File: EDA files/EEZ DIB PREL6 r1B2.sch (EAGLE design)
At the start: 65 parts, among them IC1 STM32F030C6T6, IC2 74HC1G126GW,125, IC3 M24C32-WMN6P, IC4 LP2985-33DBVR, K1 RT424005, K2 RT424005, K3 RT424005, K4 RT424005, K5 RT424005, K6 RT424005, Q1 2N7002, Q2 2N7002, Q3 2N7002, Q4 2N7002, Q5 2N7002, Q6 2N7002, X1 SSW-106-02-S-S, X2 77317-104-28LF, X3 691327310016, X4 691327310016

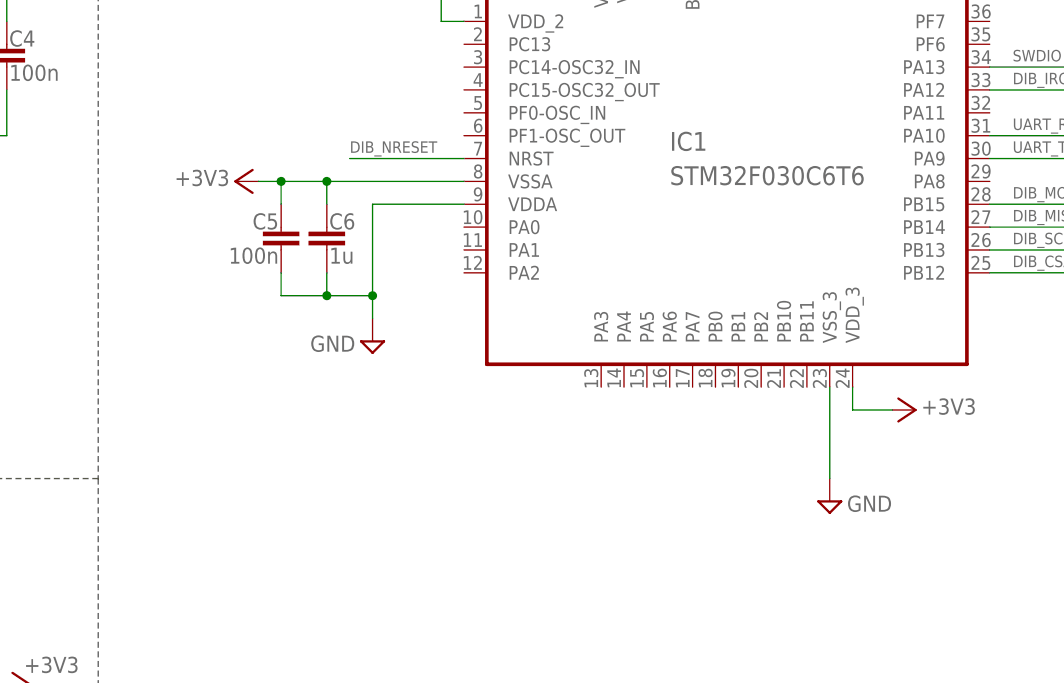
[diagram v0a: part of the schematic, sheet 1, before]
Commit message: #1 fixed
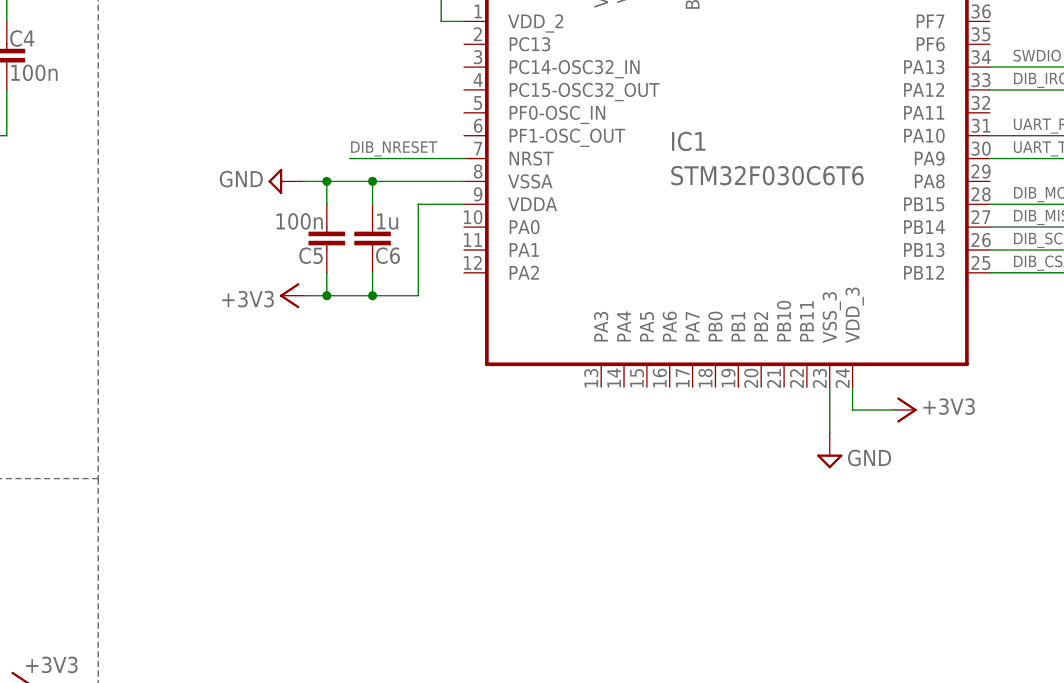
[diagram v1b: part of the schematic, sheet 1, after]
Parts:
- C2, C8, C9: device rcl:C-EUC1206 -> rcl:C-EUC0805
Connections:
- net +3V3: now also IC1.VDDA; no longer IC1.VSSA
- net GND: now also IC1.VSSA; no longer IC1.VDDA
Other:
- moved on the sheet: C5, C6
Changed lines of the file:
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@@
 <part name="SUPPLY66" library="supply2" deviceset="GND" device=""/>
 <part name="SUPPLY67" library="supply2" deviceset="GND" device=""/>
-<part name="C8" library="rcl" deviceset="C-EU" device="C1206" value="2u2"/>
+<part name="C8" library="rcl" deviceset="C-EU" device="C0805" value="2u2"/>
 <part name="P+1" library="supply1" deviceset="+5V" device=""/>
 <part name="P+2" library="supply1" deviceset="+5V" device=""/>
@@
 <part name="P+5" library="supply1" deviceset="+5V" device=""/>
 <part name="IC1" library="EEZ_DIB" deviceset="STM32F030" device="C6T6"/>
-<part name="SUPPLY48" library="supply2" deviceset="GND" device=""/>
 <part name="SUPPLY49" library="supply2" deviceset="GND" device=""/>
 <part name="C1" library="rcl" deviceset="C-EU" device="C0603" value="100n"/>
-<part name="C2" library="rcl" deviceset="C-EU" device="C1206" value="4u7"/>
+<part name="C2" library="rcl" deviceset="C-EU" device="C0805" value="4u7"/>
 <part name="SUPPLY61" library="supply2" deviceset="GND" device=""/>
 <part name="+3V4" library="supply1" deviceset="+3V3" device=""/>
@@
 <part name="C3" library="EEZ_Lib1" deviceset="ECAP" device="PANASONIC_H" value="EEEFK1V470P"/>
 <part name="SUPPLY45" library="supply2" deviceset="GND" device=""/>
-<part name="C9" library="rcl" deviceset="C-EU" device="C1206" value="4u7"/>
+<part name="C9" library="rcl" deviceset="C-EU" device="C0805" value="4u7"/>
 <part name="RN2" library="EEZ_Lib1" deviceset="R_ARRAY4" device="" value="DR1206-10K-4/8"/>
 <part name="+3V5" library="supply1" deviceset="+3V3" device=""/>
@@
 <part name="R7" library="rcl" deviceset="R-EU_" device="R0805" value="100K"/>
 <part name="X1" library="con-samtec" deviceset="SSW-106-02-S-S" device=""/>
+<part name="SUPPLY6" library="supply2" deviceset="GND" device=""/>
 </parts>
 <sheets>
@@
 <attribute name="VALUE" x="205.74" y="98.6536" size="2.0828" layer="96" ratio="6" rot="SR0"/>
 </instance>
-<instance part="SUPPLY48" gate="GND" x="172.72" y="81.28" smashed="yes">
-<attribute name="VALUE" x="170.815" y="81.915" size="1.778" layer="96" rot="R180"/>
-</instance>
-<instance part="SUPPLY49" gate="GND" x="223.52" y="63.5" smashed="yes">
-<attribute name="VALUE" x="225.425" y="64.135" size="1.778" layer="96" rot="MR180"/>
+<instance part="SUPPLY49" gate="GND" x="223.52" y="68.58" smashed="yes">
+<attribute name="VALUE" x="225.425" y="69.215" size="1.778" layer="96" rot="MR180"/>
 </instance>
 <instance part="C1" gate="G$1" x="195.58" y="144.78" smashed="yes" rot="MR90">
@@
 <attribute name="VALUE" x="248.285" y="140.335" size="1.778" layer="96" rot="MR180"/>
 </instance>
-<instance part="C6" gate="G$1" x="167.64" y="91.44" smashed="yes" rot="MR180">
-<attribute name="NAME" x="167.894" y="93.726" size="1.778" layer="95"/>
-<attribute name="VALUE" x="167.894" y="89.916" size="1.778" layer="96"/>
-</instance>
-<instance part="C5" gate="G$1" x="162.56" y="93.98" smashed="yes" rot="MR0">
-<attribute name="NAME" x="162.306" y="93.726" size="1.778" layer="95" rot="MR0"/>
-<attribute name="VALUE" x="162.306" y="89.916" size="1.778" layer="96" rot="MR0"/>
-</instance>
-<instance part="+3V2" gate="G$1" x="157.48" y="99.06" smashed="yes" rot="MR270">
-<attribute name="VALUE" x="156.845" y="100.33" size="1.778" layer="96" rot="R180"/>
+<instance part="C6" gate="G$1" x="172.72" y="93.98" smashed="yes">
+<attribute name="NAME" x="172.974" y="91.694" size="1.778" layer="95" rot="MR180"/>
+<attribute name="VALUE" x="172.974" y="95.504" size="1.778" layer="96" rot="MR180"/>
+</instance>
+<instance part="C5" gate="G$1" x="167.64" y="91.44" smashed="yes" rot="R180">
+<attribute name="NAME" x="167.386" y="91.694" size="1.778" layer="95" rot="R180"/>
+<attribute name="VALUE" x="167.386" y="95.504" size="1.778" layer="96" rot="R180"/>
+</instance>
+<instance part="+3V2" gate="G$1" x="162.56" y="86.36" smashed="yes" rot="R90">
+<attribute name="VALUE" x="161.925" y="85.09" size="1.778" layer="96" rot="MR0"/>
 </instance>
 <instance part="+3V3" gate="G$1" x="233.045" y="73.66" smashed="yes" rot="MR90">
@@
 <instance part="X1" gate="-4" x="177.8" y="165.1" smashed="yes" rot="MR0">
 <attribute name="NAME" x="180.848" y="165.862" size="1.524" layer="95" rot="MR180"/>
+</instance>
+<instance part="SUPPLY6" gate="GND" x="162.56" y="99.06" smashed="yes" rot="MR90">
+<attribute name="VALUE" x="160.655" y="98.425" size="1.778" layer="96" rot="MR0"/>
 </instance>
 </instances>
@@
 </segment>
 <segment>
-<pinref part="IC1" gate="G$1" pin="VDDA"/>
-<wire x1="182.88" y1="96.52" x2="172.72" y2="96.52" width="0.1524" layer="91"/>
-<wire x1="172.72" y1="96.52" x2="172.72" y2="86.36" width="0.1524" layer="91"/>
-<pinref part="SUPPLY48" gate="GND" pin="GND"/>
 <pinref part="C6" gate="G$1" pin="1"/>
-<wire x1="172.72" y1="86.36" x2="172.72" y2="83.82" width="0.1524" layer="91"/>
-<wire x1="172.72" y1="86.36" x2="167.64" y2="86.36" width="0.1524" layer="91"/>
-<wire x1="167.64" y1="86.36" x2="167.64" y2="88.9" width="0.1524" layer="91"/>
-<junction x="172.72" y="86.36"/>
+<wire x1="172.72" y1="99.06" x2="172.72" y2="96.52" width="0.1524" layer="91"/>
 <pinref part="C5" gate="G$1" pin="2"/>
-<wire x1="167.64" y1="86.36" x2="162.56" y2="86.36" width="0.1524" layer="91"/>
-<wire x1="162.56" y1="86.36" x2="162.56" y2="88.9" width="0.1524" layer="91"/>
-<junction x="167.64" y="86.36"/>
+<wire x1="172.72" y1="99.06" x2="167.64" y2="99.06" width="0.1524" layer="91"/>
+<wire x1="167.64" y1="99.06" x2="167.64" y2="96.52" width="0.1524" layer="91"/>
+<junction x="172.72" y="99.06"/>
+<pinref part="IC1" gate="G$1" pin="VSSA"/>
+<wire x1="172.72" y1="99.06" x2="182.88" y2="99.06" width="0.1524" layer="91"/>
+<pinref part="SUPPLY6" gate="GND" pin="GND"/>
+<wire x1="167.64" y1="99.06" x2="165.1" y2="99.06" width="0.1524" layer="91"/>
+<junction x="167.64" y="99.06"/>
 </segment>
 <segment>
 <pinref part="IC1" gate="G$1" pin="VSS_3"/>
-<wire x1="223.52" y1="76.2" x2="223.52" y2="66.04" width="0.1524" layer="91"/>
+<wire x1="223.52" y1="76.2" x2="223.52" y2="71.12" width="0.1524" layer="91"/>
 <pinref part="SUPPLY49" gate="GND" pin="GND"/>
 </segment>
@@
 </segment>
 <segment>
-<pinref part="IC1" gate="G$1" pin="VSSA"/>
-<wire x1="182.88" y1="99.06" x2="167.64" y2="99.06" width="0.1524" layer="91"/>
 <pinref part="C6" gate="G$1" pin="2"/>
-<wire x1="167.64" y1="99.06" x2="167.64" y2="96.52" width="0.1524" layer="91"/>
+<wire x1="172.72" y1="86.36" x2="172.72" y2="88.9" width="0.1524" layer="91"/>
 <pinref part="C5" gate="G$1" pin="1"/>
-<wire x1="167.64" y1="99.06" x2="162.56" y2="99.06" width="0.1524" layer="91"/>
-<wire x1="162.56" y1="99.06" x2="162.56" y2="96.52" width="0.1524" layer="91"/>
-<junction x="167.64" y="99.06"/>
-<wire x1="162.56" y1="99.06" x2="160.02" y2="99.06" width="0.1524" layer="91"/>
-<junction x="162.56" y="99.06"/>
+<wire x1="172.72" y1="86.36" x2="167.64" y2="86.36" width="0.1524" layer="91"/>
+<wire x1="167.64" y1="86.36" x2="167.64" y2="88.9" width="0.1524" layer="91"/>
+<wire x1="167.64" y1="86.36" x2="165.1" y2="86.36" width="0.1524" layer="91"/>
+<junction x="167.64" y="86.36"/>
 <pinref part="+3V2" gate="G$1" pin="+3V3"/>
-</segment>
-<segment>
+<pinref part="IC1" gate="G$1" pin="VDDA"/>
+<wire x1="182.88" y1="96.52" x2="177.8" y2="96.52" width="0.1524" layer="91"/>
+<wire x1="177.8" y1="96.52" x2="177.8" y2="86.36" width="0.1524" layer="91"/>
+<wire x1="177.8" y1="86.36" x2="172.72" y2="86.36" width="0.1524" layer="91"/>
+<junction x="172.72" y="86.36"/>
+</segment>
+<segment>
